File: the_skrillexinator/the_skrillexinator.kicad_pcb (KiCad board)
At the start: 2 copper layers, 3 parts, among them J1 Conn_01x03, J2 Conn_01x03, U1 ESP32-WROOM-32

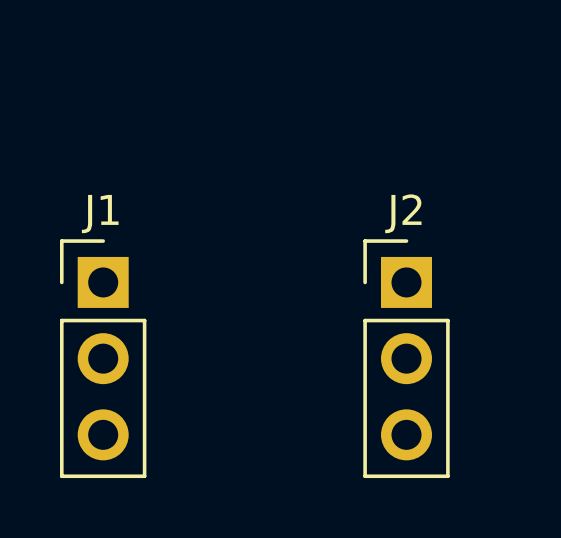
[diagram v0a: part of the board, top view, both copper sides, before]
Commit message: skibidi
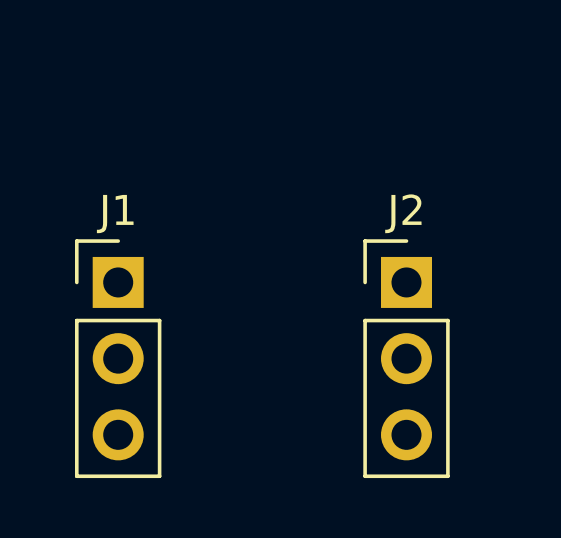
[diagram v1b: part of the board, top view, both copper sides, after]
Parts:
- moved J1 0.50 mm to (107.0, 91.7)
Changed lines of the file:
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@@
 	(footprint "Connector_PinHeader_2.54mm:PinHeader_1x03_P2.54mm_Vertical"
 		(layer "F.Cu")
-		(at 106.5 91.65)
+		(at 107 91.65)
 		(descr "Through hole straight pin header, 1x03, 2.54mm pitch, single row")
 		(tags "Through hole pin header THT 1x03 2.54mm single row")
